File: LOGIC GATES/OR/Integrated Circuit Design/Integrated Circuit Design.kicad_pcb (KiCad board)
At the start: 2 copper layers, 25 x 40 mm, 0 parts

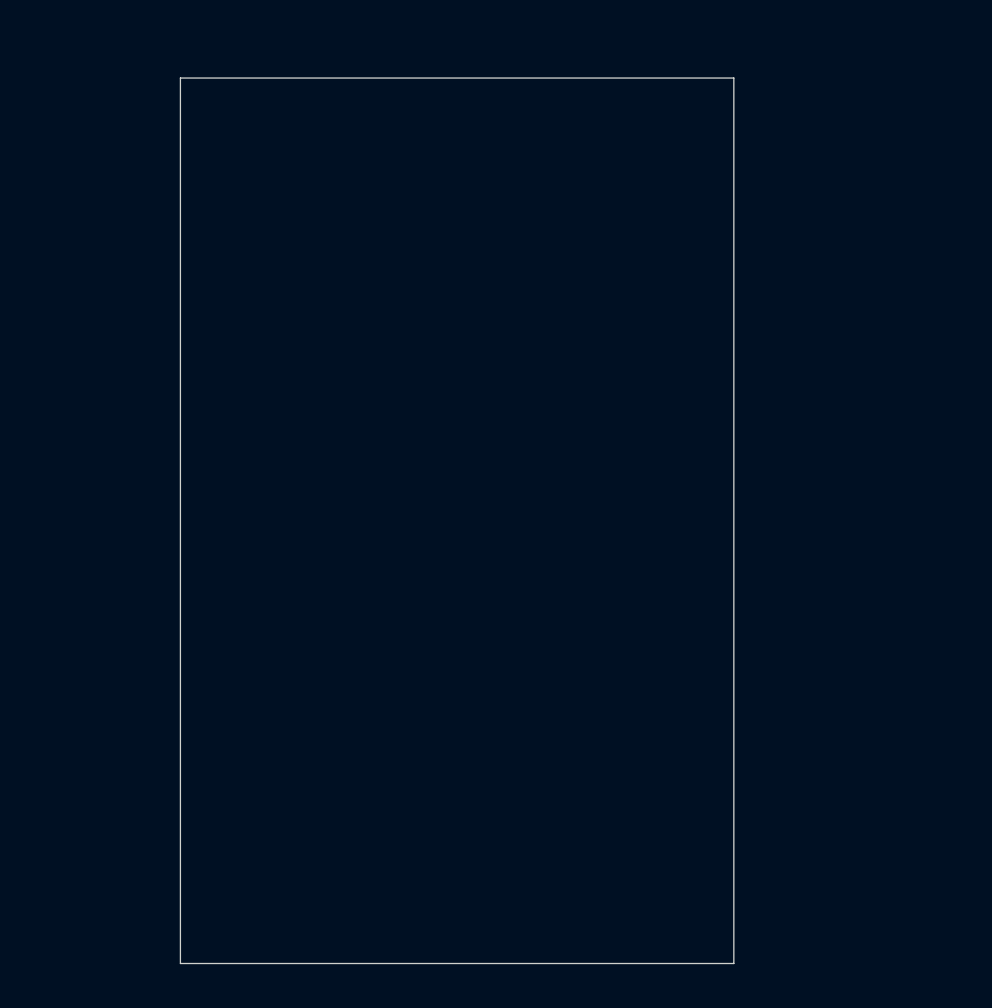
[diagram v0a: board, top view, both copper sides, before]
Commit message: Auto-update: 22.12.2025 16:16:21,18
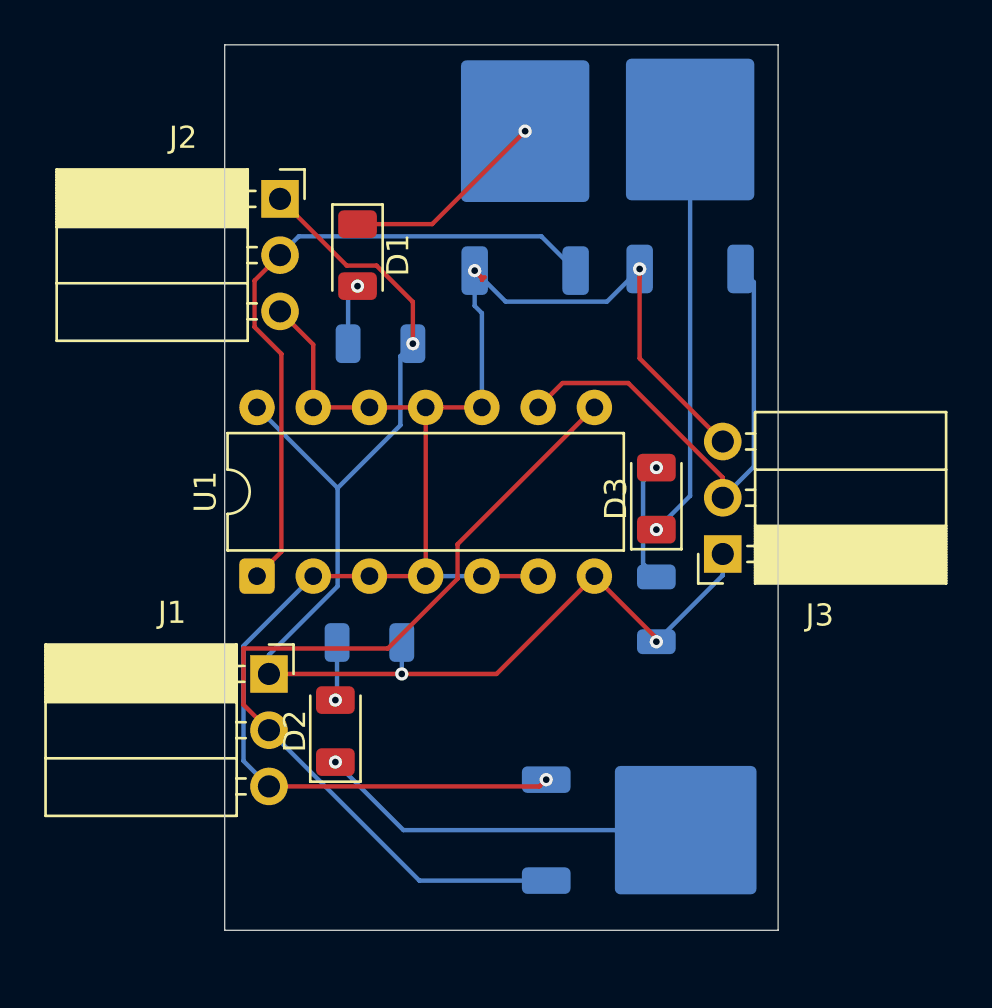
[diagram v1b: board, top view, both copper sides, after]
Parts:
- added D1: LED, LED_SMD:LED_1206_3216Metric, F.Cu at (116.0, 84.5)
- added D2: LED, LED_SMD:LED_1206_3216Metric, F.Cu at (115.0, 106.0)
- added D3: LED, LED_SMD:LED_1206_3216Metric, F.Cu at (129.5, 95.5)
- added J1: Conn_01x03_Socket, Connector_PinSocket_2.54mm:PinSocket_1x03_P2.54mm_Horizontal, F.Cu at (112.0, 103.4)
- added J2: Conn_01x03_Socket, Connector_PinSocket_2.54mm:PinSocket_1x03_P2.54mm_Horizontal, F.Cu at (112.5, 82.0)
- added J3: Conn_01x03_Socket, Connector_PinSocket_2.54mm:PinSocket_1x03_P2.54mm_Horizontal, F.Cu at (132.5, 98.0)
- added Q1: QM6006D, Package_TO_SOT_SMD:TO-252-2, B.Cu at (123.6, 80.2)
- added Q2: QM6006D, Package_TO_SOT_SMD:TO-252-2, B.Cu at (129.6, 110.5)
- added Q3: QM6006D, Package_TO_SOT_SMD:TO-252-2, B.Cu at (131.0, 80.1)
- added R1: R, Resistor_SMD:R_1206_3216Metric, B.Cu at (117.0, 88.5)
- added R2: R, Resistor_SMD:R_1206_3216Metric, B.Cu at (116.5, 102.0)
- added R3: R, Resistor_SMD:R_1206_3216Metric, B.Cu at (129.5, 100.5)
- added U1: 4075, Package_DIP:DIP-14_W7.62mm, F.Cu at (111.5, 99.0)
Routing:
- net Net-(J1-Pin_3): track 0.00 -> 79.3 mm, vias 0 -> 3
- net Net-(J1-Pin_1): track 0.00 -> 59.9 mm, vias 0 -> 3
- net Net-(J1-Pin_2): track 0.00 -> 40.8 mm
- net Net-(J2-Pin_2): track 0.00 -> 30.3 mm
- net Net-(J3-Pin_2): track 0.00 -> 22.6 mm
- net Net-(D3-K): track 0.00 -> 18.7 mm, vias 0 -> 1
- net Net-(D2-K): track 0.00 -> 17.1 mm, vias 0 -> 1
- net Net-(D1-K): track 0.00 -> 9.31 mm, vias 0 -> 1
- net Net-(D3-A): track 0.00 -> 5.44 mm, vias 0 -> 1
- net Net-(D1-A): track 0.00 -> 2.78 mm, vias 0 -> 1
- net Net-(D2-A): track 0.00 -> 2.63 mm, vias 0 -> 1
